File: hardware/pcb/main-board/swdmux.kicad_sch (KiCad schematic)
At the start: 2 parts, among them U901 MUX

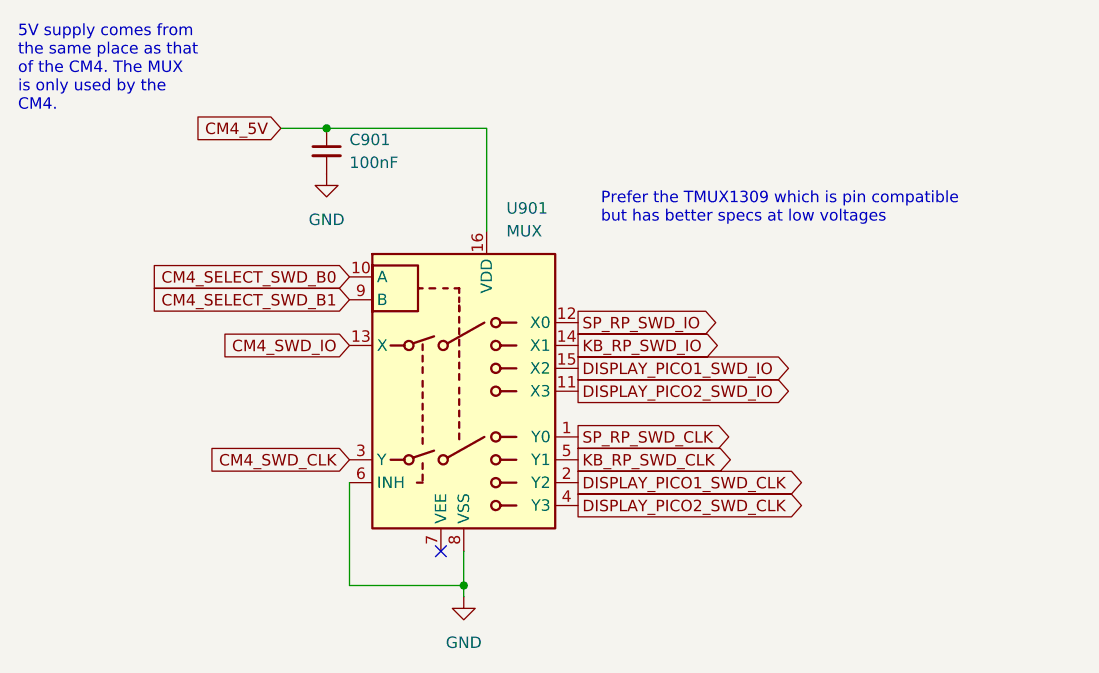
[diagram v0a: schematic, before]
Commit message: tidy the keyboard comms
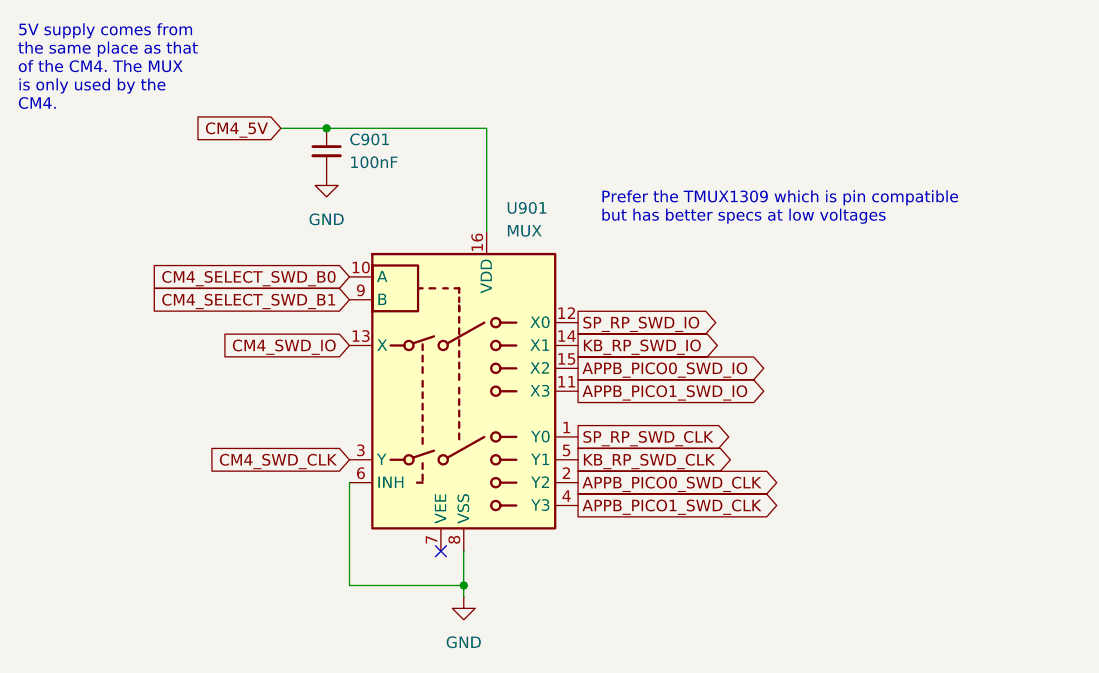
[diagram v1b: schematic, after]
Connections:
- net DISPLAY_PICO1_SWD_CLK renamed APPB_PICO0_SWD_CLK
- net DISPLAY_PICO1_SWD_IO renamed APPB_PICO0_SWD_IO
- net DISPLAY_PICO2_SWD_CLK renamed APPB_PICO1_SWD_CLK
- net DISPLAY_PICO2_SWD_IO renamed APPB_PICO1_SWD_IO
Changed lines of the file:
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@@
 		)
 	)
-	(global_label "DISPLAY_PICO1_SWD_CLK"
+	(global_label "APPB_PICO0_SWD_CLK"
 		(shape output)
 		(at 96.52 83.82 0)
@@
 		)
 		(property "Intersheetrefs" "${INTERSHEET_REFS}"
-			(at 122.4972 83.82 0)
+			(at 119.8362 83.82 0)
 			(effects
 				(font
@@
 		)
 	)
-	(global_label "DISPLAY_PICO2_SWD_IO"
+	(global_label "APPB_PICO1_SWD_IO"
 		(shape output)
 		(at 96.52 73.66 0)
@@
 		)
 		(property "Intersheetrefs" "${INTERSHEET_REFS}"
-			(at 120.8644 73.66 0)
+			(at 118.2034 73.66 0)
 			(effects
 				(font
@@
 		)
 	)
-	(global_label "DISPLAY_PICO2_SWD_CLK"
+	(global_label "APPB_PICO1_SWD_CLK"
 		(shape output)
 		(at 96.52 86.36 0)
@@
 		)
 		(property "Intersheetrefs" "${INTERSHEET_REFS}"
-			(at 122.4972 86.36 0)
+			(at 119.8362 86.36 0)
 			(effects
 				(font
@@
 		)
 	)
-	(global_label "DISPLAY_PICO1_SWD_IO"
+	(global_label "APPB_PICO0_SWD_IO"
 		(shape output)
 		(at 96.52 71.12 0)
@@
 		)
 		(property "Intersheetrefs" "${INTERSHEET_REFS}"
-			(at 120.8644 71.12 0)
+			(at 118.2034 71.12 0)
 			(effects
 				(font
